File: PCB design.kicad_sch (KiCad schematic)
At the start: 10 parts, among them U1 STM32F205RBTx

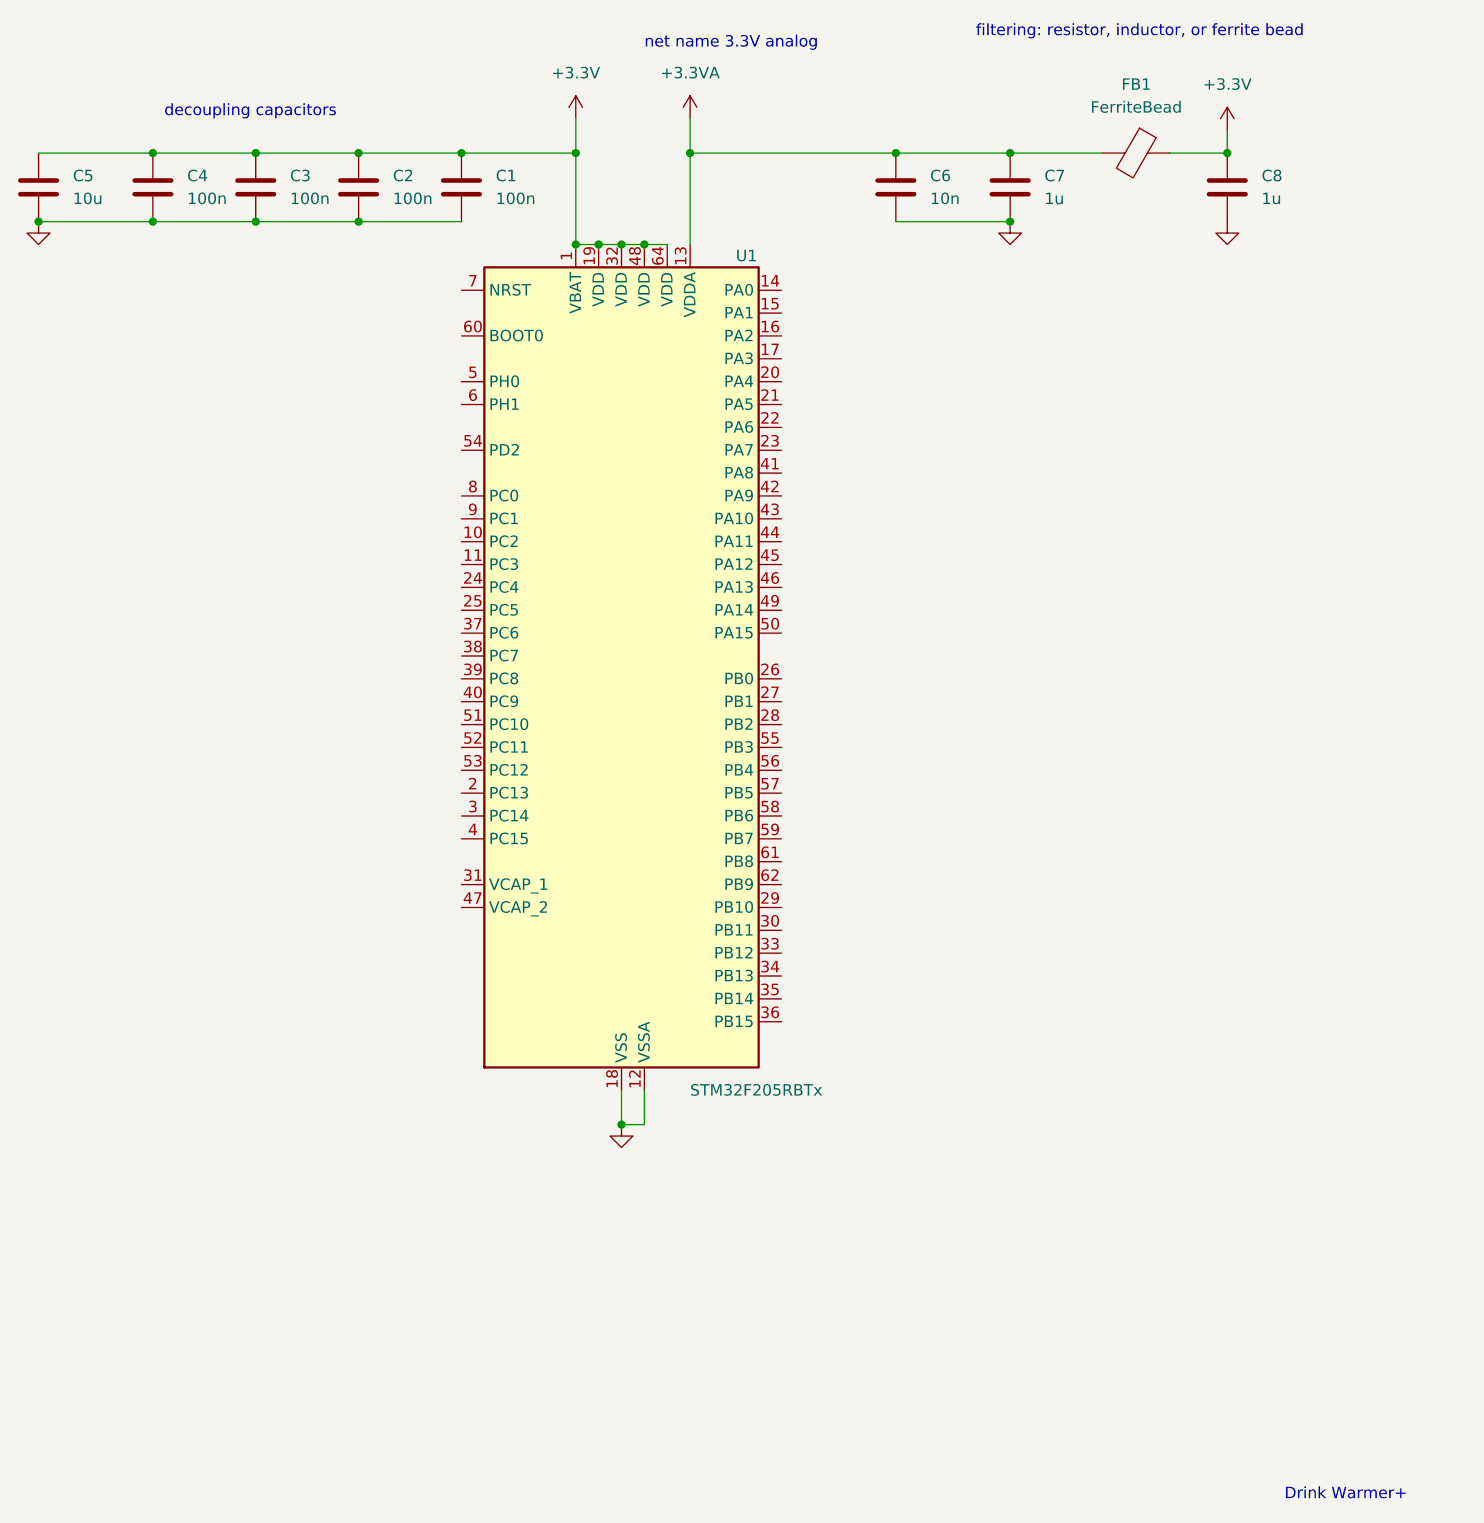
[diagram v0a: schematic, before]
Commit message: Add files via upload
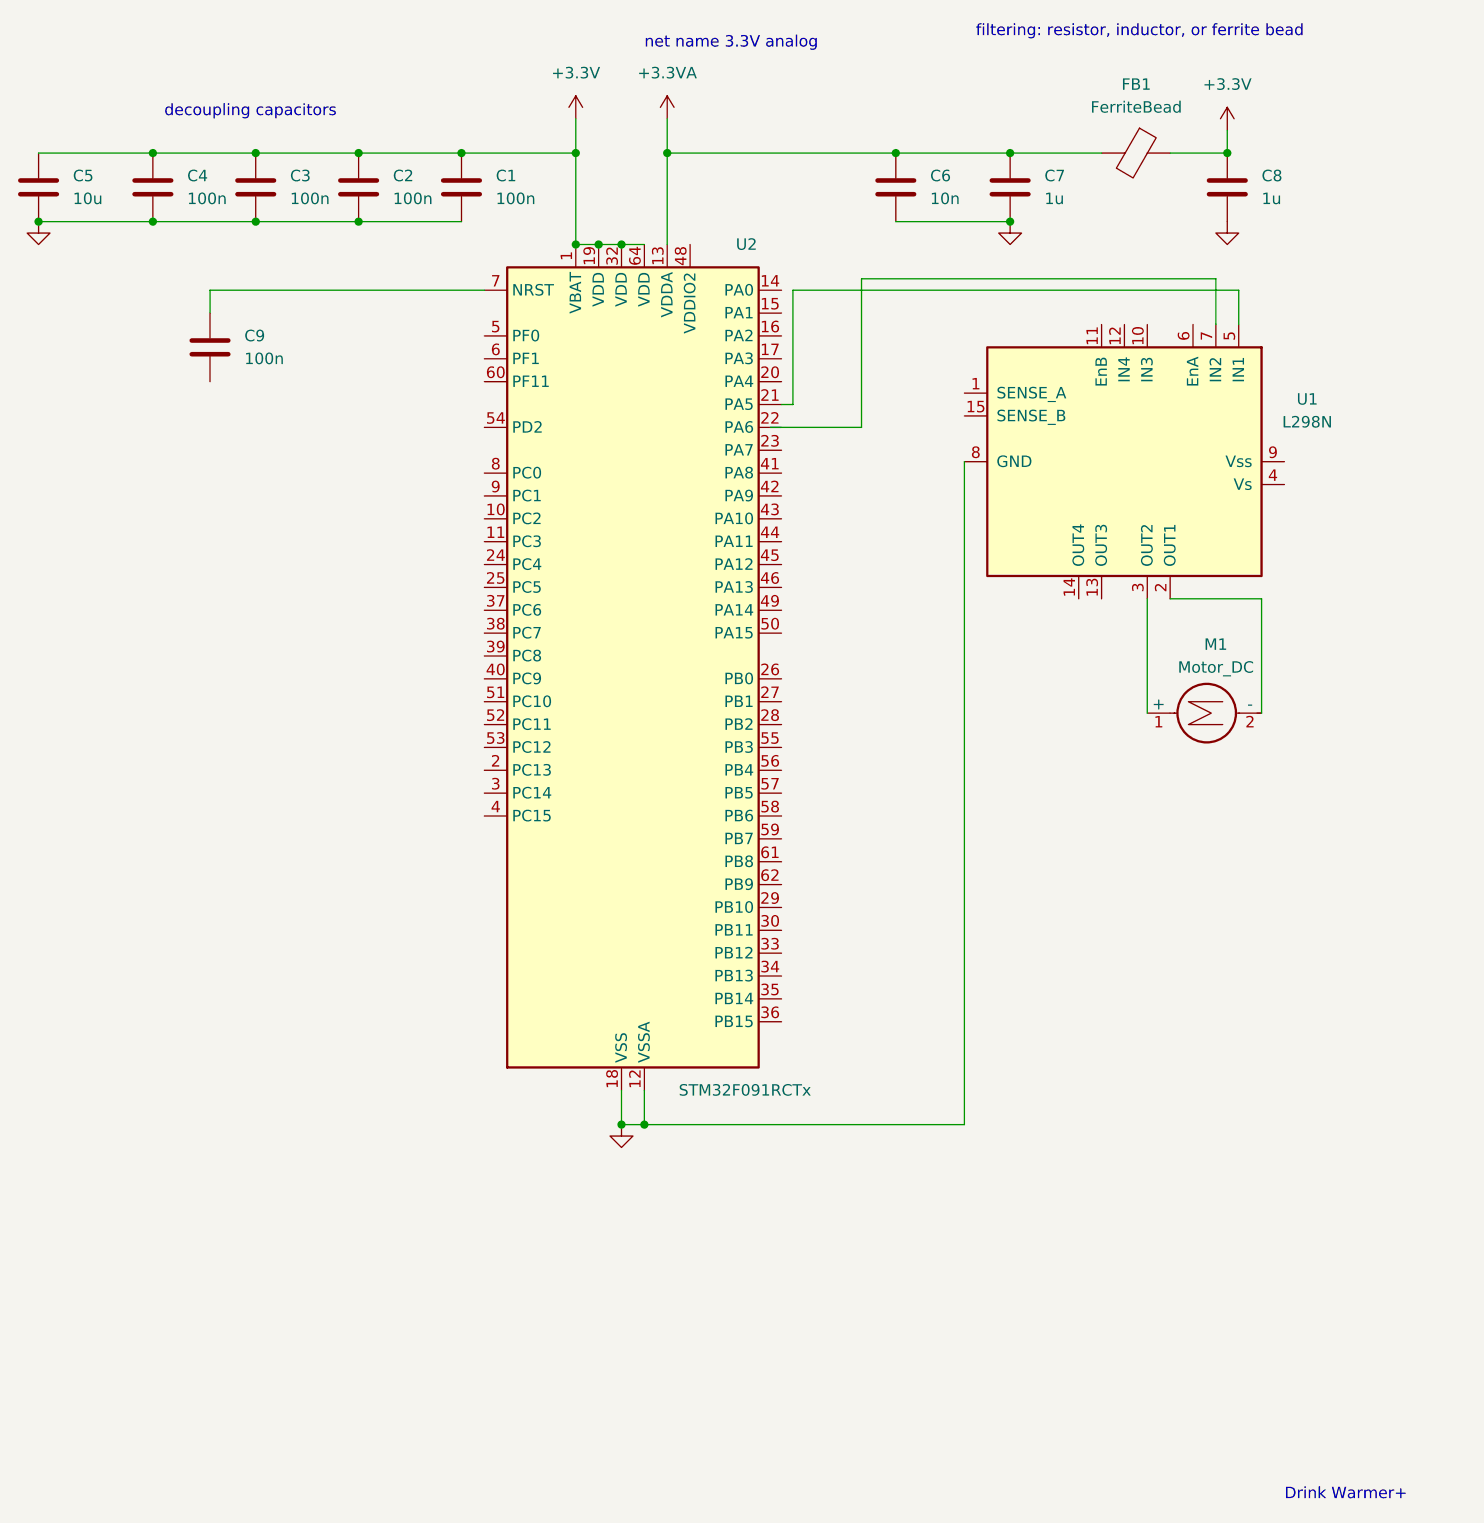
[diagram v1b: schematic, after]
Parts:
- removed U1: STM32F205RBTx, Package_QFP:LQFP-64_10x10mm_P0.5mm, symbol MCU_ST_STM32F2:STM32F205RBTx
- added C9: 100n, symbol Device:C
- added M1: Motor_DC, symbol Motor:Motor_DC
- added U1: L298N, Package_TO_SOT_THT:TO-220-15_P2.54x2.54mm_StaggerOdd_Lead4.58mm_Vertical, symbol Driver_Motor:L298N
- added U2: STM32F091RCTx, Package_QFP:LQFP-64_10x10mm_P0.5mm, symbol MCU_ST_STM32F0:STM32F091RCTx
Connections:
- net +3.3V: now also U2.1 (VBAT), U2.19 (VDD), U2.32 (VDD), U2.64 (VDD)
- net +3.3VA: now also U2.13 (VDDA)
- net GND: now also U1.8 (GND), U2.12 (VSSA), U2.18 (VSS), U2.31 (VSS), U2.47 (VSS), U2.63 (VSS)
- new net: C9.1, U2.7 (NRST)
- new net: U1.5 (IN1), U2.21 (PA5)
- new net: M1.1 (+), U1.3 (OUT2)
- new net: M1.2 (-), U1.2 (OUT1)
